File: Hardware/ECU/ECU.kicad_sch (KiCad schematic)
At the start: 4 parts, among them U1 Teensy4.1

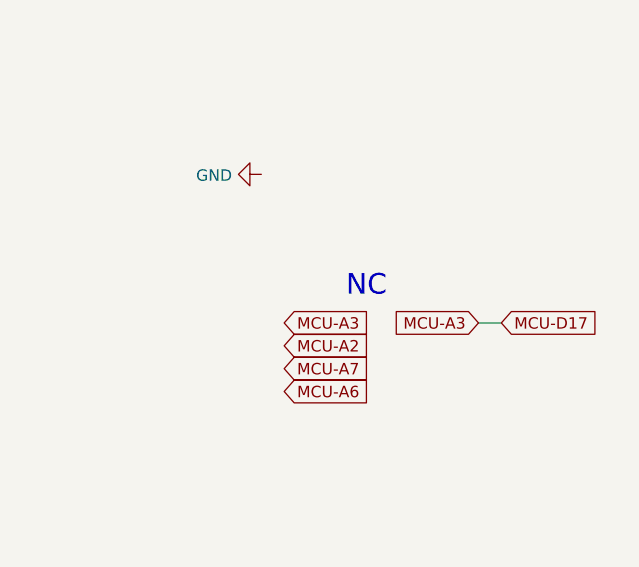
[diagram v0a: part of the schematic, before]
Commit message: renamed:    Hardware/ECU/ECU-backups/ECU-2025-05-27_141528.zip -> Hardware/ECU/ECU-backups/ECU-2025-05-27_234640.zip 	renamed:    Hardware/ECU/ECU-backups/ECU-2025-05-27_154948.zip -> Hardware/ECU/ECU-backups/ECU-2025-05-27_235240.zip 	modified:   Hardware/ECU/ECU.kicad_pcb 	modified:   Hardware/ECU/ECU.kicad_prl 	modified:   Hardware/ECU/ECU.kicad_sch
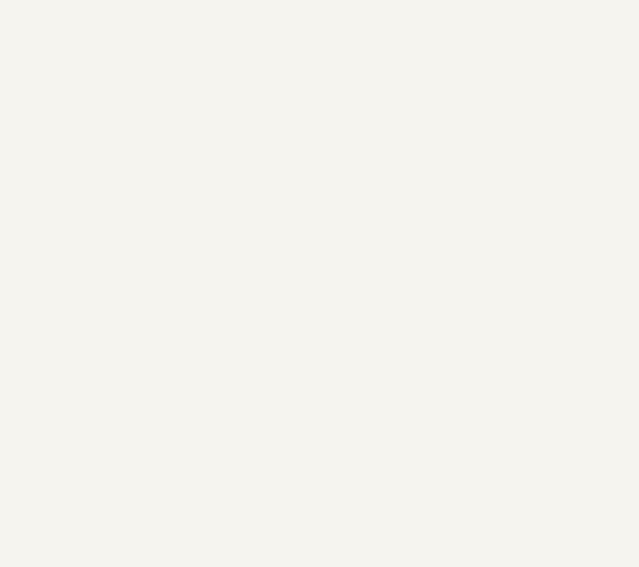
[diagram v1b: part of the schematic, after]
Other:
- note removed: "NC"

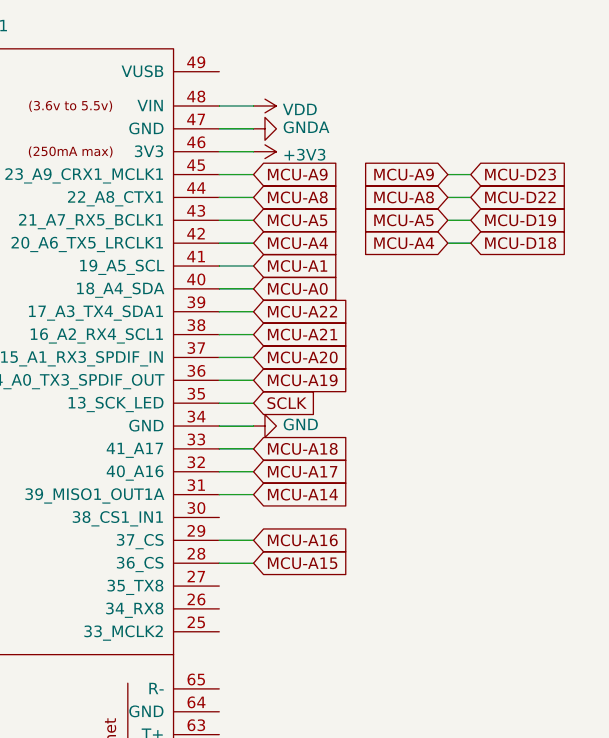
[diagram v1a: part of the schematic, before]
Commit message: deleted:    Hardware/ECU/ECU-backups/ECU-2025-05-27_235240.zip 	deleted:    Hardware/ECU/ECU-backups/ECU-2025-05-28_135321.zip 	deleted:    Hardware/ECU/ECU-backups/ECU-2025-05-28_140049.zip 	deleted:    Hardware/ECU/ECU-backups/ECU-2025-05-28_141416.zip 	deleted:    Hardware/ECU/ECU-backups/ECU-2025-05-28_154718.zip 	deleted:    Hardware/ECU/ECU-backups/ECU-2025-06-18_111329.zip 	new file:   Hardware/ECU/ECU-backups/ECU-2025-08-26_154141.zip 	new file:   Hardware/ECU/ECU-backups/ECU-2025-08-29_143817.zip 	new file:   Hardware/ECU/ECU-backups/ECU-2025-09-19_081818.zip 	new file:   Hardware/ECU/ECU-backups/ECU-2026-01-19_151411.zip 	new file:   Hardware/ECU/ECU-backups/ECU-2026-01-19_152057.zip 	new file:   Hardware/ECU/ECU-backups/ECU-2026-01-19_154705.zip 	modified:   Hardware/ECU/ECU.kicad_pcb 	modified:   Hardware/ECU/ECU.kicad_prl 	modified:   Hardware/ECU/ECU.kicad_sch 	modified:   Hardware/ECU/Inputs.kicad_sch 	modified:   Hardware/ECU/Inputs2.kicad_sch 	renamed:    Hardware/ECU/output/PCB.pdf -> Hardware/ECU/output/PCB-R9.3.pdf 	renamed:    Hardware/ECU/output/Schematics.pdf -> Hardware/ECU/output/Schematics-R0.3.pdf 	new file:   Hardware/ECU/output/Schematics-R1.pdf 	deleted:    Hardware/ECU/output/cut files/ECU-B_Cu.jpg 	modified:   speeduino (modified content)
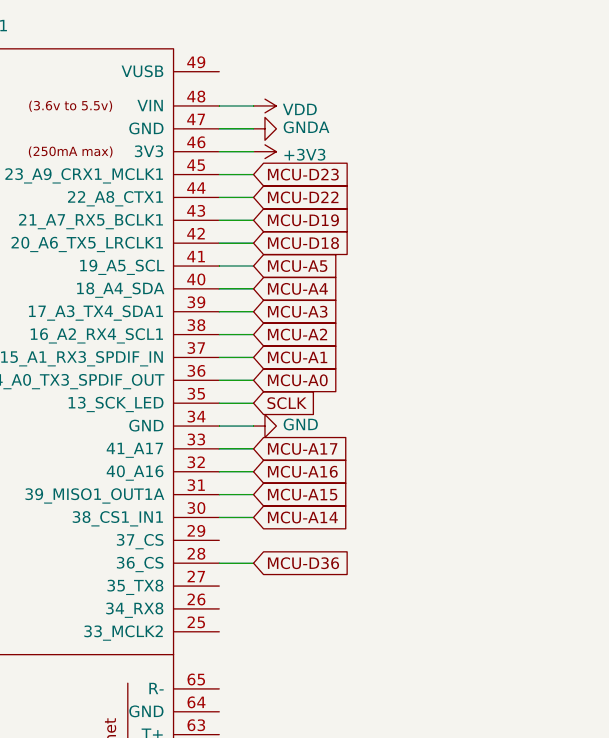
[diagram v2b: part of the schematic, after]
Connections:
- net MCU-A18 is gone; now on net MCU-A17: U1.33 (41_A17)
- net MCU-A19 is gone; now on net MCU-A0: U1.36 (14_A0_TX3_SPDIF_OUT)
- net MCU-A20 is gone; now on net MCU-A1: U1.37 (15_A1_RX3_SPDIF_IN)
- net MCU-A0: no longer U1.40 (18_A4_SDA)
- net MCU-A1: no longer U1.41 (19_A5_SCL)
- net MCU-A14: now also U1.30 (38_CS1_IN1); no longer U1.31 (39_MISO1_OUT1A)
- net MCU-A15: now also U1.31 (39_MISO1_OUT1A); no longer U1.28 (36_CS)
- net MCU-A16: now also U1.32 (40_A16); no longer U1.29 (37_CS)
- net MCU-A17: no longer U1.32 (40_A16)
- net MCU-A4: now also U1.40 (18_A4_SDA); no longer U1.42 (20_A6_TX5_LRCLK1)
- net MCU-A5: now also U1.41 (19_A5_SCL); no longer U1.43 (21_A7_RX5_BCLK1)
- net MCU-A21 renamed MCU-A2
- net MCU-A22 renamed MCU-A3
- net MCU-A8 renamed MCU-D22
- net MCU-A9 renamed MCU-D23
- new net MCU-D18: U1.42 (20_A6_TX5_LRCLK1)
- new net MCU-D19: U1.43 (21_A7_RX5_BCLK1)
- new net MCU-D36: U1.28 (36_CS)
